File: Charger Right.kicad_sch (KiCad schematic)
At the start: 24 parts, among them J2 BRAUNIT, Q3 AO4459, Q4 2N7002, Q6 2N7002, U2 CN3702

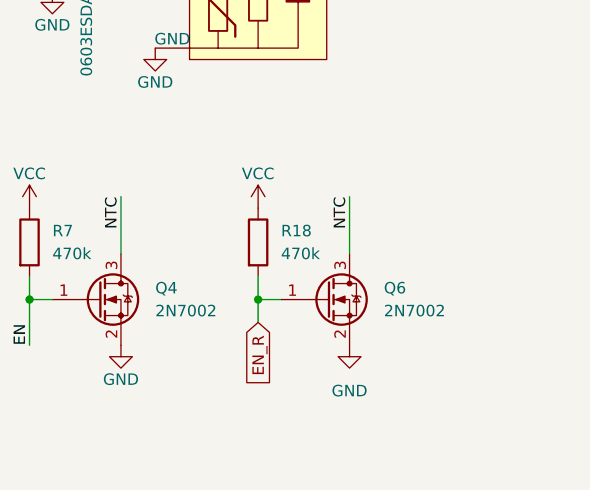
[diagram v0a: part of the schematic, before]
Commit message: WIP traces
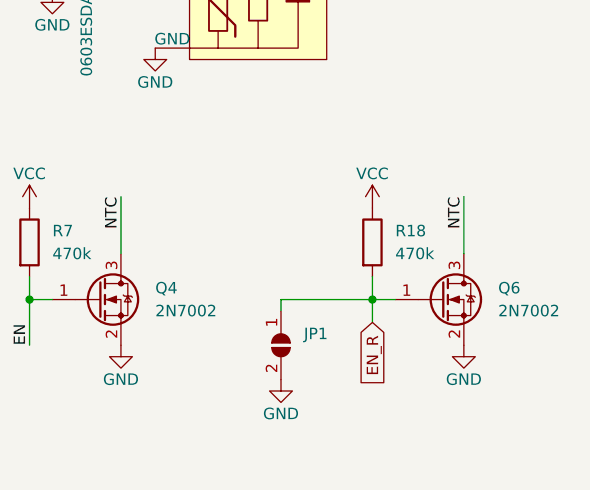
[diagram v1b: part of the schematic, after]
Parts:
- added JP1: SolderJumper_2_Open, Jumper:SolderJumper-2_P1.3mm_Open_TrianglePad1.0x1.5mm, symbol Jumper:SolderJumper_2_Open
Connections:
- net EN_R: now also JP1.1 (A)
- net GND: now also JP1.2 (B)
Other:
- moved on the sheet: Q6, R18
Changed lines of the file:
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@@
   (junction (at 138.43 123.19) (diameter 0) (color 0 0 0 0)
   )
-  (junction (at 208.28 114.3) (diameter 0) (color 0 0 0 0)
+  (junction (at 220.98 114.3) (diameter 0) (color 0 0 0 0)
   )
   (junction (at 185.42 72.39) (diameter 0) (color 0 0 0 0)
@@
     (stroke (width 0) (type default) (color 0 0 0 0))
   )
-  (wire (pts (xy 208.28 114.3) (xy 210.82 114.3))
+  (wire (pts (xy 220.98 114.3) (xy 223.52 114.3))
     (stroke (width 0) (type default) (color 0 0 0 0))
   )
@@
     (stroke (width 0) (type default) (color 0 0 0 0))
   )
+  (wire (pts (xy 210.82 114.3) (xy 220.98 114.3))
+    (stroke (width 0) (type default) (color 0 0 0 0))
+  )
   (wire (pts (xy 138.43 123.19) (xy 149.86 123.19))
     (stroke (width 0) (type default) (color 0 0 0 0))
@@
     (stroke (width 0) (type default) (color 0 0 0 0))
   )
-  (wire (pts (xy 218.44 102.87) (xy 218.44 109.22))
-    (stroke (width 0) (type default) (color 0 0 0 0))
-  )
-  (wire (pts (xy 208.28 111.76) (xy 208.28 114.3))
+  (wire (pts (xy 231.14 102.87) (xy 231.14 109.22))
+    (stroke (width 0) (type default) (color 0 0 0 0))
+  )
+  (wire (pts (xy 220.98 111.76) (xy 220.98 114.3))
     (stroke (width 0) (type default) (color 0 0 0 0))
   )
@@
     (stroke (width 0) (type default) (color 0 0 0 0))
   )
-  (wire (pts (xy 208.28 114.3) (xy 208.28 116.84))
+  (wire (pts (xy 220.98 114.3) (xy 220.98 116.84))
+    (stroke (width 0) (type default) (color 0 0 0 0))
+  )
+  (wire (pts (xy 210.82 115.57) (xy 210.82 114.3))
     (stroke (width 0) (type default) (color 0 0 0 0))
   )
@@
     (effects (font (size 1.27 1.27)) (justify left bottom))
   )
-  (label "NTC" (at 218.44 102.87 270)
+  (label "NTC" (at 231.14 102.87 270)
     (effects (font (size 1.27 1.27)) (justify right bottom))
   )
@@
     (effects (font (size 1.27 1.27)) (justify left bottom))
   )
-  (global_label "EN_R" (shape input) (at 208.28 116.84 270) (fields_autoplaced)
+  (global_label "EN_R" (shape input) (at 220.98 116.84 270) (fields_autoplaced)
     (effects (font (size 1.27 1.27)) (justify right))
-    (property "Intersheet References" "${INTERSHEET_REFS}" (id 0) (at 208.2006 123.9702 90)
+    (property "Intersheet References" "${INTERSHEET_REFS}" (id 0) (at 220.9006 123.9702 90)
       (effects (font (size 1.27 1.27)) (justify right) hide)
     )
   )
-  (symbol (lib_id "power:VCC") (at 208.28 104.14 0) (unit 1)
-    (in_bom yes) (on_board yes)
-    (property "Reference" "#PWR0135" (id 0) (at 208.28 107.95 0)
-      (effects (font (size 1.27 1.27)) hide)
-    )
-    (property "Value" "VCC" (id 1) (at 208.28 100.33 0))
-    (property "Footprint" "" (id 2) (at 208.28 104.14 0)
-      (effects (font (size 1.27 1.27)) hide)
-    )
-    (property "Datasheet" "" (id 3) (at 208.28 104.14 0)
+  (symbol (lib_id "power:VCC") (at 220.98 104.14 0) (unit 1)
+    (in_bom yes) (on_board yes)
+    (property "Reference" "#PWR0135" (id 0) (at 220.98 107.95 0)
+      (effects (font (size 1.27 1.27)) hide)
+    )
+    (property "Value" "VCC" (id 1) (at 220.98 100.33 0))
+    (property "Footprint" "" (id 2) (at 220.98 104.14 0)
+      (effects (font (size 1.27 1.27)) hide)
+    )
+    (property "Datasheet" "" (id 3) (at 220.98 104.14 0)
       (effects (font (size 1.27 1.27)) hide)
     )
@@
     (pin "2")
   )
+  (symbol (lib_id "power:GND") (at 210.82 123.19 0) (unit 1)
+    (in_bom yes) (on_board yes)
+    (property "Reference" "#PWR?" (id 0) (at 210.82 129.54 0)
+      (effects (font (size 1.27 1.27)) hide)
+    )
+    (property "Value" "GND" (id 1) (at 210.82 127 0))
+    (property "Footprint" "" (id 2) (at 210.82 123.19 0)
+      (effects (font (size 1.27 1.27)) hide)
+    )
+    (property "Datasheet" "" (id 3) (at 210.82 123.19 0)
+      (effects (font (size 1.27 1.27)) hide)
+    )
+    (pin "1")
+  )
   (symbol (lib_id "power:GND") (at 124.46 128.27 0) (unit 1)
     (in_bom yes) (on_board yes)
@@
     (pin "2")
   )
-  (symbol (lib_id "Device:R") (at 208.28 107.95 0) (unit 1)
-    (in_bom yes) (on_board yes) (fields_autoplaced)
-    (property "Reference" "R18" (id 0) (at 210.82 106.6799 0)
-      (effects (font (size 1.27 1.27)) (justify left))
-    )
-    (property "Value" "470k" (id 1) (at 210.82 109.2199 0)
-      (effects (font (size 1.27 1.27)) (justify left))
-    )
-    (property "Footprint" "Resistor_SMD:R_0603_1608Metric" (id 2) (at 206.502 107.95 90)
-      (effects (font (size 1.27 1.27)) hide)
-    )
-    (property "Datasheet" "~" (id 3) (at 208.28 107.95 0)
-      (effects (font (size 1.27 1.27)) hide)
-    )
-    (property "LCSC" "C114622" (id 4) (at 208.28 107.95 0)
+  (symbol (lib_id "Device:R") (at 220.98 107.95 0) (unit 1)
+    (in_bom yes) (on_board yes) (fields_autoplaced)
+    (property "Reference" "R18" (id 0) (at 223.52 106.6799 0)
+      (effects (font (size 1.27 1.27)) (justify left))
+    )
+    (property "Value" "470k" (id 1) (at 223.52 109.2199 0)
+      (effects (font (size 1.27 1.27)) (justify left))
+    )
+    (property "Footprint" "Resistor_SMD:R_0603_1608Metric" (id 2) (at 219.202 107.95 90)
+      (effects (font (size 1.27 1.27)) hide)
+    )
+    (property "Datasheet" "~" (id 3) (at 220.98 107.95 0)
+      (effects (font (size 1.27 1.27)) hide)
+    )
+    (property "LCSC" "C114622" (id 4) (at 220.98 107.95 0)
       (effects (font (size 1.27 1.27)) hide)
     )
@@
     )
     (pin "1")
+  )
+  (symbol (lib_id "Jumper:SolderJumper_2_Open") (at 210.82 119.38 270) (unit 1)
+    (in_bom yes) (on_board yes) (fields_autoplaced)
+    (property "Reference" "JP1" (id 0) (at 213.36 118.1099 90)
+      (effects (font (size 1.27 1.27)) (justify left))
+    )
+    (property "Value" "SolderJumper_2_Open" (id 1) (at 213.36 120.6499 90)
+      (effects (font (size 1.27 1.27)) (justify left) hide)
+    )
+    (property "Footprint" "Jumper:SolderJumper-2_P1.3mm_Open_TrianglePad1.0x1.5mm" (id 2) (at 210.82 119.38 0)
+      (effects (font (size 1.27 1.27)) hide)
+    )
+    (property "Datasheet" "~" (id 3) (at 210.82 119.38 0)
+      (effects (font (size 1.27 1.27)) hide)
+    )
+    (pin "1")
+    (pin "2")
   )
   (symbol (lib_id "Device:R_Shunt") (at 158.75 72.39 90) (mirror x) (unit 1)
@@
     (pin "3")
   )
-  (symbol (lib_id "Transistor_FET:2N7002") (at 215.9 114.3 0) (unit 1)
-    (in_bom yes) (on_board yes) (fields_autoplaced)
-    (property "Reference" "Q6" (id 0) (at 222.25 113.0299 0)
-      (effects (font (size 1.27 1.27)) (justify left))
-    )
-    (property "Value" "2N7002" (id 1) (at 222.25 115.5699 0)
-      (effects (font (size 1.27 1.27)) (justify left))
-    )
-    (property "Footprint" "Package_TO_SOT_SMD:SOT-23" (id 2) (at 220.98 116.205 0)
+  (symbol (lib_id "Transistor_FET:2N7002") (at 228.6 114.3 0) (unit 1)
+    (in_bom yes) (on_board yes) (fields_autoplaced)
+    (property "Reference" "Q6" (id 0) (at 234.95 113.0299 0)
+      (effects (font (size 1.27 1.27)) (justify left))
+    )
+    (property "Value" "2N7002" (id 1) (at 234.95 115.5699 0)
+      (effects (font (size 1.27 1.27)) (justify left))
+    )
+    (property "Footprint" "Package_TO_SOT_SMD:SOT-23" (id 2) (at 233.68 116.205 0)
       (effects (font (size 1.27 1.27) italic) (justify left) hide)
     )
-    (property "Datasheet" "https://www.onsemi.com/pub/Collateral/NDS7002A-D.PDF" (id 3) (at 215.9 114.3 0)
+    (property "Datasheet" "https://www.onsemi.com/pub/Collateral/NDS7002A-D.PDF" (id 3) (at 228.6 114.3 0)
       (effects (font (size 1.27 1.27)) (justify left) hide)
     )
-    (property "LCSC" "C8545" (id 4) (at 215.9 114.3 0)
+    (property "LCSC" "C8545" (id 4) (at 228.6 114.3 0)
       (effects (font (size 1.27 1.27)) hide)
     )
@@
     (pin "2")
   )
-  (symbol (lib_id "power:GND") (at 218.44 119.38 0) (unit 1)
-    (in_bom yes) (on_board yes) (fields_autoplaced)
-    (property "Reference" "#PWR0136" (id 0) (at 218.44 125.73 0)
-      (effects (font (size 1.27 1.27)) hide)
-    )
-    (property "Value" "GND" (id 1) (at 218.44 124.46 0))
-    (property "Footprint" "" (id 2) (at 218.44 119.38 0)
-      (effects (font (size 1.27 1.27)) hide)
-    )
-    (property "Datasheet" "" (id 3) (at 218.44 119.38 0)
-      (effects (font (size 1.27 1.27)) hide)
-    )
+  (symbol (lib_id "power:GND") (at 231.14 119.38 0) (unit 1)
+    (in_bom yes) (on_board yes)
+    (property "Reference" "#PWR0136" (id 0) (at 231.14 125.73 0)
+      (effects (font (size 1.27 1.27)) hide)
+    )
+    (property "Value" "GND" (id 1) (at 231.14 123.19 0))
+    (property "Footprint" "" (id 2) (at 231.14 119.38 0)
+      (effects (font (size 1.27 1.27)) hide)
+    )
+    (property "Datasheet" "" (id 3) (at 231.14 119.38 0)
+      (effects (font (size 1.27 1.27)) hide)
+    )
